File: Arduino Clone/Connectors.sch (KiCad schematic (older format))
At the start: 4 parts

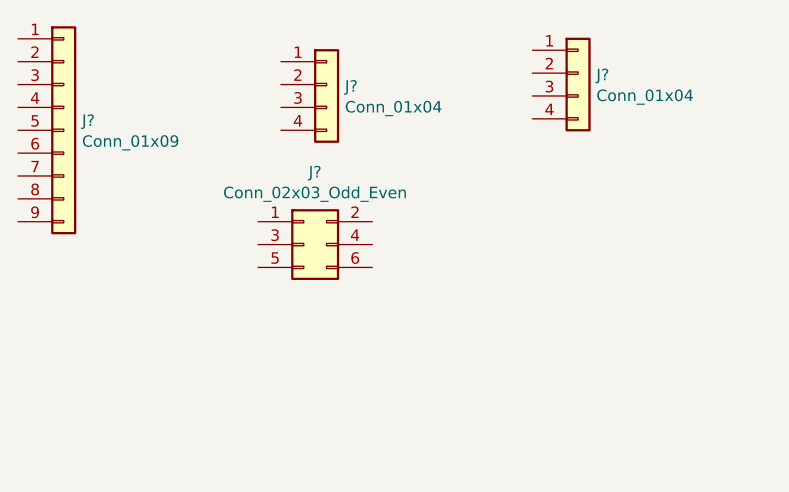
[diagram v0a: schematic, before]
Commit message: 30%
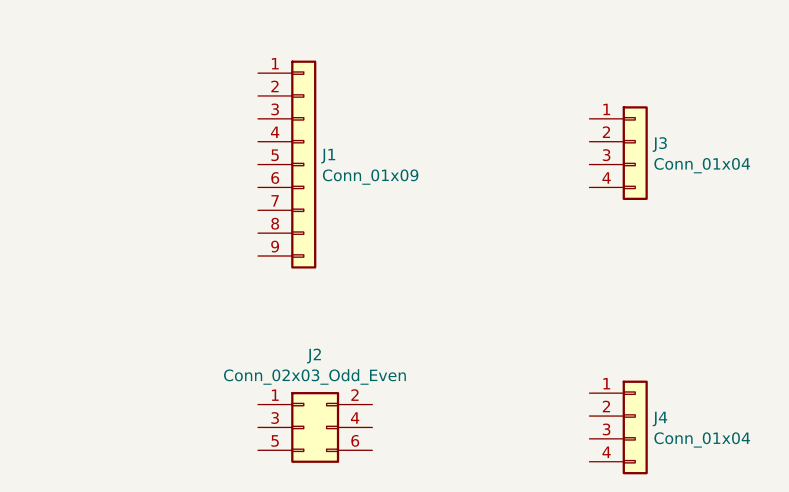
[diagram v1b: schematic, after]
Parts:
- J1: renamed from J?; footprint (none) -> Connector_PinHeader_2.54mm:PinHeader_1x09_P2.54mm_Vertical
- J2: renamed from J?; footprint (none) -> Connector_PinHeader_2.54mm:PinHeader_2x03_P2.54mm_Vertical
- J3, J4: renamed from J?; footprint (none) -> Connector_PinHeader_2.54mm:PinHeader_1x04_P2.54mm_Vertical
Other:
- moved on the sheet: J1, J2, J3, J4
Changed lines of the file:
@@
 $EndDescr
 $Comp
-L Connector_Generic:Conn_01x09 J?
+L Connector_Generic:Conn_01x09 J1
 U 1 1 5FCF0074
-P 3850 3050
-F 0 "J?" H 3930 3092 50  0000 L CNN
-F 1 "Conn_01x09" H 3930 3001 50  0000 L CNN
-F 2 "" H 3850 3050 50  0001 C CNN
-F 3 "~" H 3850 3050 50  0001 C CNN
-	1    3850 3050
+P 4900 3200
+F 0 "J1" H 4980 3242 50  0000 L CNN
+F 1 "Conn_01x09" H 4980 3151 50  0000 L CNN
+F 2 "Connector_PinHeader_2.54mm:PinHeader_1x09_P2.54mm_Vertical" H 4900 3200 50  0001 C CNN
+F 3 "~" H 4900 3200 50  0001 C CNN
+	1    4900 3200
 	1    0    0    -1
 $EndComp
 $Comp
-L Connector_Generic:Conn_01x04 J?
+L Connector_Generic:Conn_01x04 J3
 U 1 1 5FCF0AC0
-P 5000 2850
-F 0 "J?" H 5080 2842 50  0000 L CNN
-F 1 "Conn_01x04" H 5080 2751 50  0000 L CNN
-F 2 "" H 5000 2850 50  0001 C CNN
-F 3 "~" H 5000 2850 50  0001 C CNN
-	1    5000 2850
+P 6350 3100
+F 0 "J3" H 6430 3092 50  0000 L CNN
+F 1 "Conn_01x04" H 6430 3001 50  0000 L CNN
+F 2 "Connector_PinHeader_2.54mm:PinHeader_1x04_P2.54mm_Vertical" H 6350 3100 50  0001 C CNN
+F 3 "~" H 6350 3100 50  0001 C CNN
+	1    6350 3100
 	1    0    0    -1
 $EndComp
 $Comp
-L Connector_Generic:Conn_02x03_Odd_Even J?
+L Connector_Generic:Conn_02x03_Odd_Even J2
 U 1 1 5FCF0EFC
-P 4900 3550
-F 0 "J?" H 4950 3867 50  0000 C CNN
-F 1 "Conn_02x03_Odd_Even" H 4950 3776 50  0000 C CNN
-F 2 "" H 4900 3550 50  0001 C CNN
-F 3 "~" H 4900 3550 50  0001 C CNN
-	1    4900 3550
+P 4900 4350
+F 0 "J2" H 4950 4667 50  0000 C CNN
+F 1 "Conn_02x03_Odd_Even" H 4950 4576 50  0000 C CNN
+F 2 "Connector_PinHeader_2.54mm:PinHeader_2x03_P2.54mm_Vertical" H 4900 4350 50  0001 C CNN
+F 3 "~" H 4900 4350 50  0001 C CNN
+	1    4900 4350
 	1    0    0    -1
 $EndComp
 $Comp
-L Connector_Generic:Conn_01x04 J?
+L Connector_Generic:Conn_01x04 J4
 U 1 1 5FCF1C90
-P 6100 2800
-F 0 "J?" H 6180 2792 50  0000 L CNN
-F 1 "Conn_01x04" H 6180 2701 50  0000 L CNN
-F 2 "" H 6100 2800 50  0001 C CNN
-F 3 "~" H 6100 2800 50  0001 C CNN
-	1    6100 2800
+P 6350 4300
+F 0 "J4" H 6430 4292 50  0000 L CNN
+F 1 "Conn_01x04" H 6430 4201 50  0000 L CNN
+F 2 "Connector_PinHeader_2.54mm:PinHeader_1x04_P2.54mm_Vertical" H 6350 4300 50  0001 C CNN
+F 3 "~" H 6350 4300 50  0001 C CNN
+	1    6350 4300
 	1    0    0    -1
 $EndComp
